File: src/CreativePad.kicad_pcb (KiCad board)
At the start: 2 copper layers, 66 parts, among them SW2 TS342A2P-WZ, U1 TPMIC5219-2.8YM5, U17 RP2040_C2961140, U19 W25Q128JWPIQ, U2 AMS1117-3.3, X2 DSX321G-12MHZ

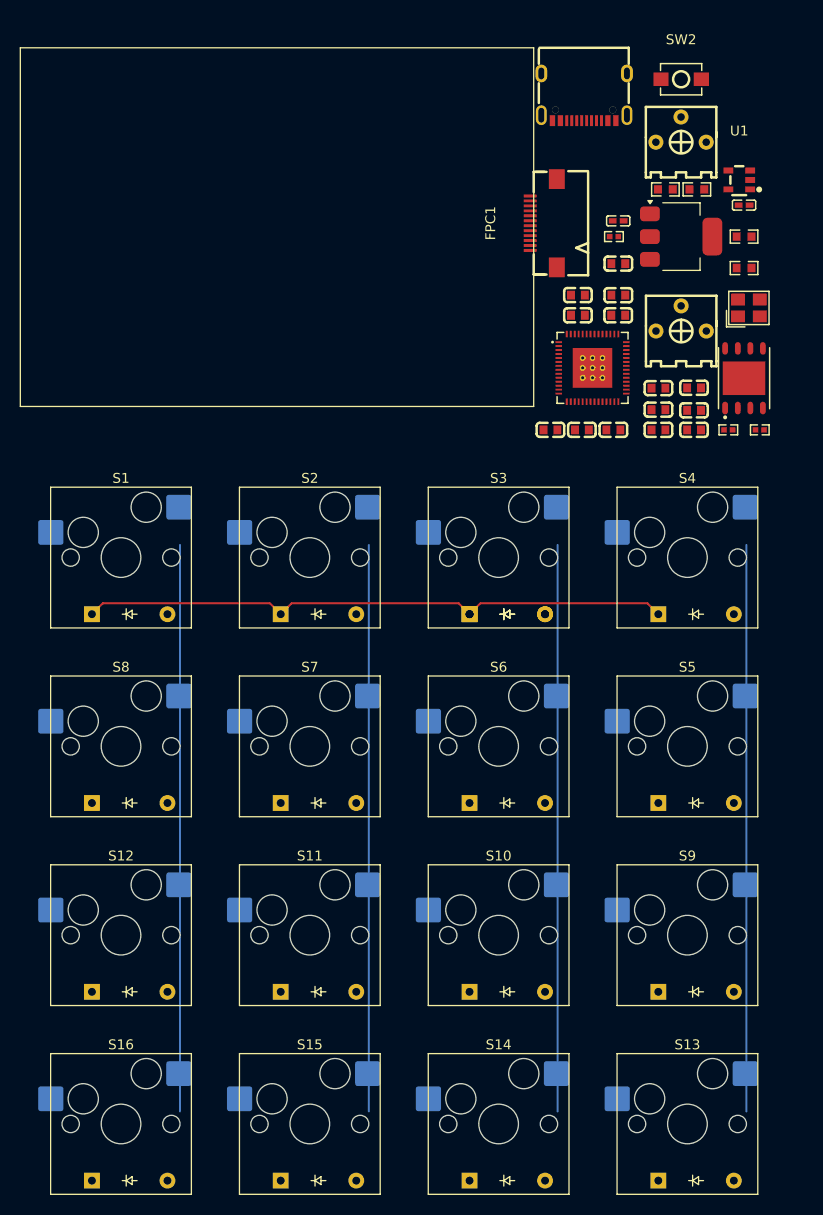
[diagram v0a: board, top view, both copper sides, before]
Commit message: Day 6
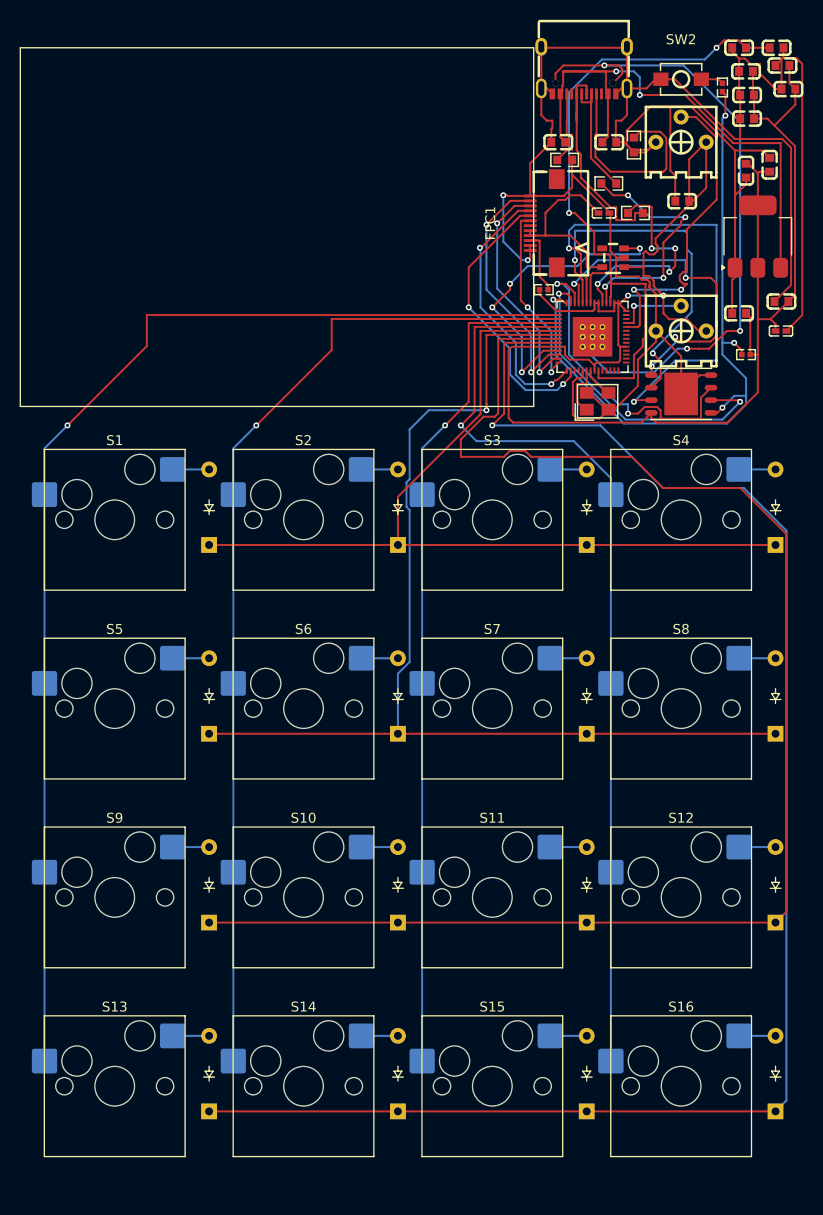
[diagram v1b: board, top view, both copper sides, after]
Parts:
- removed the D3 at (69.3, 83.7) (x2)
- added D3: Diode, ScottoKeebs_Components:Diode_DO-35, F.Cu at (81.1, 76.7)
- U17: value RP2040_C2961140 -> RP2040
- X2: value DSX321G-12MHZ -> 12MHZ
- moved S13 57.9 mm to (33.5, 131.3)
- moved S5 57.9 mm to (33.5, 93.2)
- moved S9 57.9 mm to (33.5, 112.3)
- moved S12 56.6 mm to (90.6, 112.3)
- moved S16 56.6 mm to (90.6, 131.3)
- moved S8 56.6 mm to (90.6, 93.2)
- moved C14 43.6 mm to (100.8, 28.4)
- moved C17 43.3 mm to (100.2, 26.6), turned to 180 degrees
- moved C11 36.4 mm to (97.3, 31.3), turned to 180 degrees
- moved C8 35.7 mm to (101.4, 30.7)
- moved C9 29.0 mm to (99.5, 38.4), turned to -90 degrees
- moved C1 28.8 mm to (78.2, 36.1)
- moved C7 28.2 mm to (97.2, 28.9)
- moved R8 26.0 mm to (76.7, 51.0)
- moved C2 25.3 mm to (83.4, 36.1), turned to 180 degrees
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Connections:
- S1 pad 1: (no net) -> ROW0
- S1 pad 2: (no net) -> Net-(D1-A)
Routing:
- net GND: track 0.00 -> 257.5 mm, vias 0 -> 2
- net +3V3: track 0.00 -> 176.6 mm, vias 0 -> 2
- net COL3: track 0.00 -> 165.0 mm, vias 0 -> 1
- net COL2: track 0.00 -> 153.6 mm
- net ROW0: track 0.00 -> 121.1 mm, vias 0 -> 1
- net COL1: track 0.00 -> 112.1 mm, vias 0 -> 1
- net ROW1: track 0.00 -> 101.9 mm, vias 0 -> 1
- net ROW3: track 0.00 -> 95.2 mm, vias 0 -> 1
- net ROW2: track 0.00 -> 85.5 mm, vias 0 -> 1
- net QSS: track 0.00 -> 70.2 mm, vias 0 -> 4
- net +1V1: track 0.00 -> 69.7 mm, vias 0 -> 2
- net (no net): track 0.00 -> 65.9 mm, vias 0 -> 3
- net +5V: track 0.00 -> 58.6 mm, vias 0 -> 2
- net Net-(D8-A): track 57.1 -> 3.68 mm
- net Net-(D7-A): track 57.1 -> 3.68 mm
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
